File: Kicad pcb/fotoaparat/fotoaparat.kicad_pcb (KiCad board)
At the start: 2 copper layers, 100 x 69 mm, 43 parts, among them J1 Conn_02x01, J2 Conn_01x02_Socket, Q1 BC547, Q2 BC547, Q3 BC547, Q4 BC547, SW1 SW_Push_Dual, U1 TP4056, U10 VBsemi SI2312CDS-T1-GE3, U11 VBsemi SI2312CDS-T1-GE3, U12 VBsemi SI2312CDS-T1-GE3, U2 ov7670 fifo, U3 Stm32 Bluepill, U4 Lcd Display, U5 VBsemi SI2312CDS-T1-GE3, U6 Me6211c, U7 VBsemi SI2312CDS-T1-GE3, U8 Me6211c, U9 Me6211c

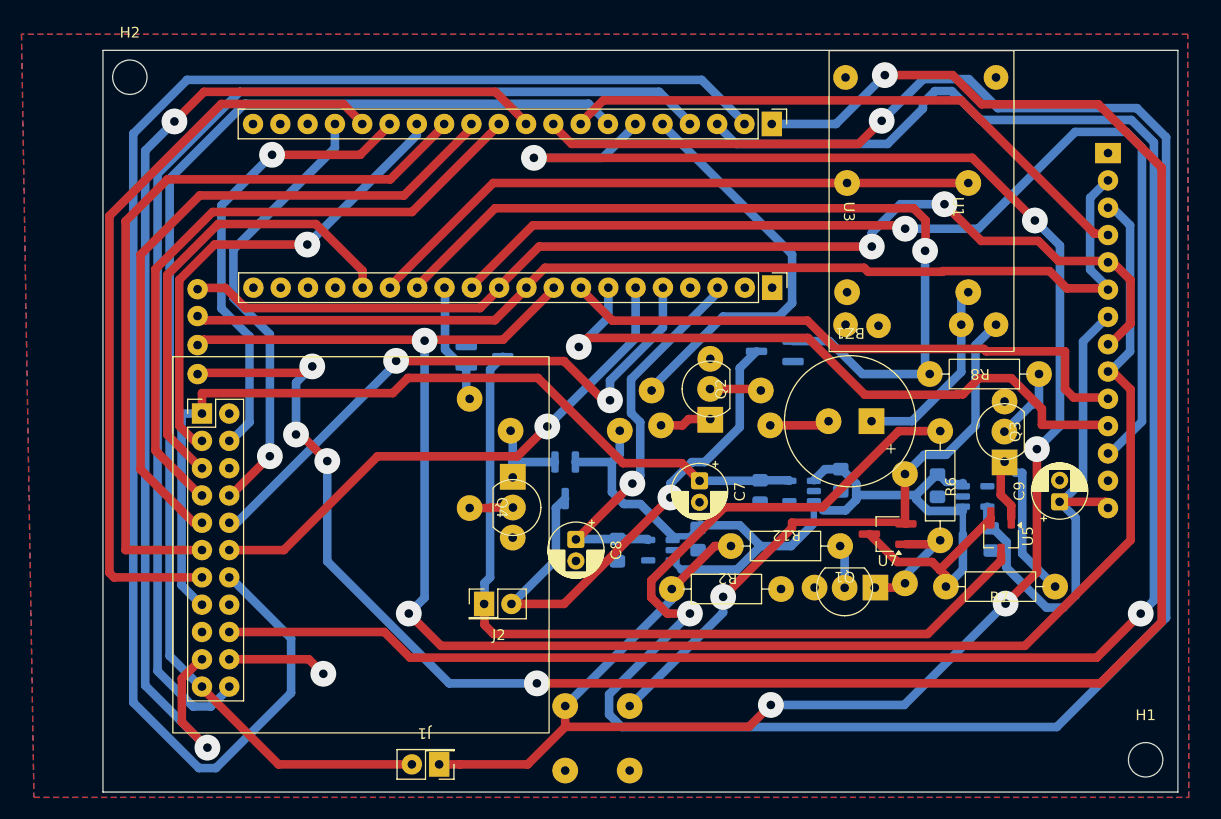
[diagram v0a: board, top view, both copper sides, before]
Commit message: Zarovnání
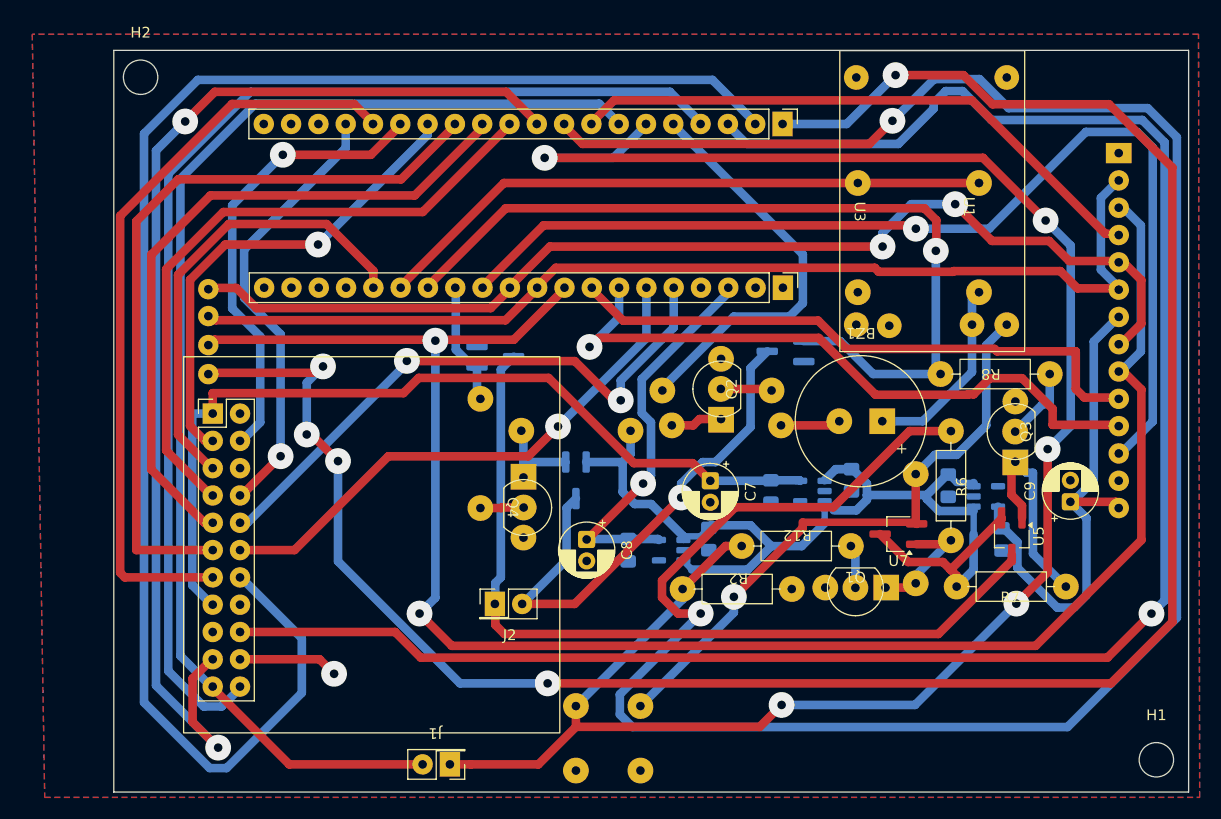
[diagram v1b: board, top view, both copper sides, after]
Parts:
- moved BZ1 1.00 mm to (69.5, -43.2)
- moved C1 1.00 mm to (55.4, -23.5)
- moved C2 1.00 mm to (47.9, -22.5)
- moved C3 1.00 mm to (68.6, -29.0)
- moved C4 1.00 mm to (61.1, -28.0)
- moved C5 1.00 mm to (77.6, -28.5)
- moved C6 1.00 mm to (82.6, -23.5)
- moved C7 1.00 mm to (55.5, -29.0)
- moved C8 1.00 mm to (44.0, -23.5)
- moved C9 1.00 mm to (89.0, -27.0)
- moved H1 1.00 mm to (97.0, -3.00)
- moved H2 1.00 mm to (2.50, -66.5)
- moved J1 1.00 mm to (29.9, -5.97)
- moved J2 1.00 mm to (36.8, -14.1)
- moved Q1 1.00 mm to (69.0, -20.5)
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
